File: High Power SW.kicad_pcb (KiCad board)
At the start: 2 copper layers, 48 x 36 mm, 21 parts, among them CN1 Jumper_NC_Small, Q1 PSMN5R6-60YLX, U1 PS2801C-1-A

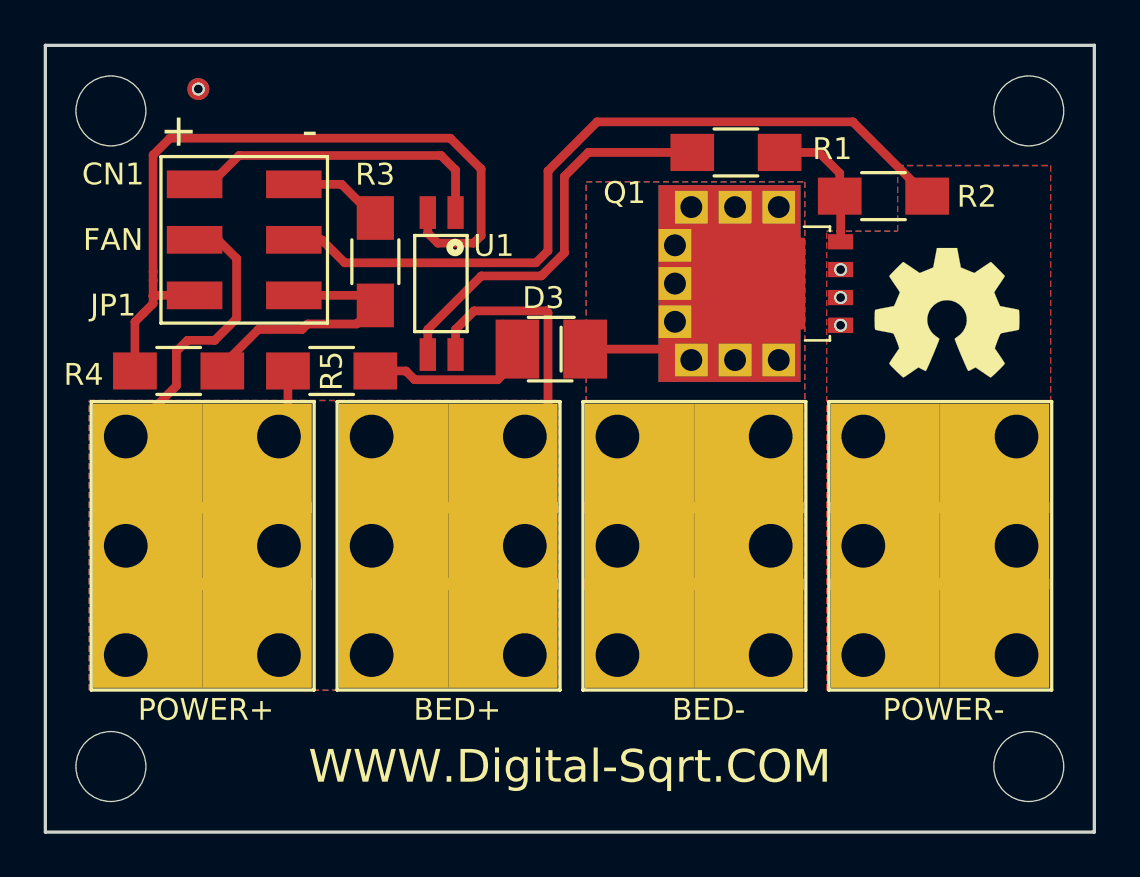
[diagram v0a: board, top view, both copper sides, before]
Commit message: Updtes for Manufacture
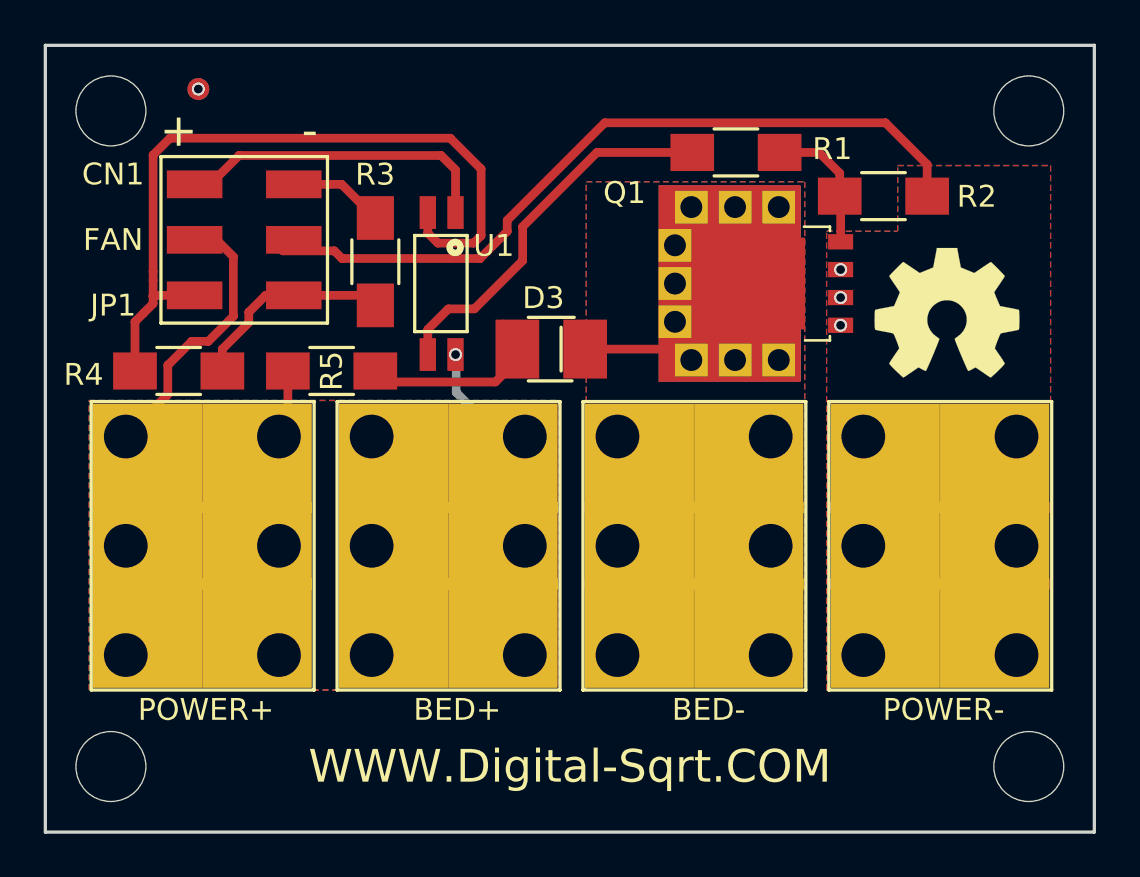
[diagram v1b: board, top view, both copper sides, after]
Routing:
- net +BATT: track 28.3 -> 23.3 mm, vias 0 -> 1
- net Net-(JP1-Pad2): track 13.3 -> 9.93 mm
- net GND: track 38.4 -> 37.3 mm
- net Net-(R1-Pad1): track 18.7 -> 17.5 mm
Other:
- net class Default: clearance 0.2 -> 0.3048
- net class Power: clearance 0.2 -> 0.3048
- net class small_trace: clearance 0.2 -> 0.3048
- rule trace_clearance: 0.2 -> 0.3048
